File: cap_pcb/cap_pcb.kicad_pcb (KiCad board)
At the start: 2 copper layers, 43 parts, among them U0 ATtiny85-20PU, U1 PCF8574, U10 HDSP-7803, U11 HDSP-7803, U12 PCF8574, U2 HDSP-7803, U3 PCF8574, U4 HDSP-7803, U5 PCF8574, U6 HDSP-7803, U7 PCF8574, U8 HDSP-7803, U9 PCF8574

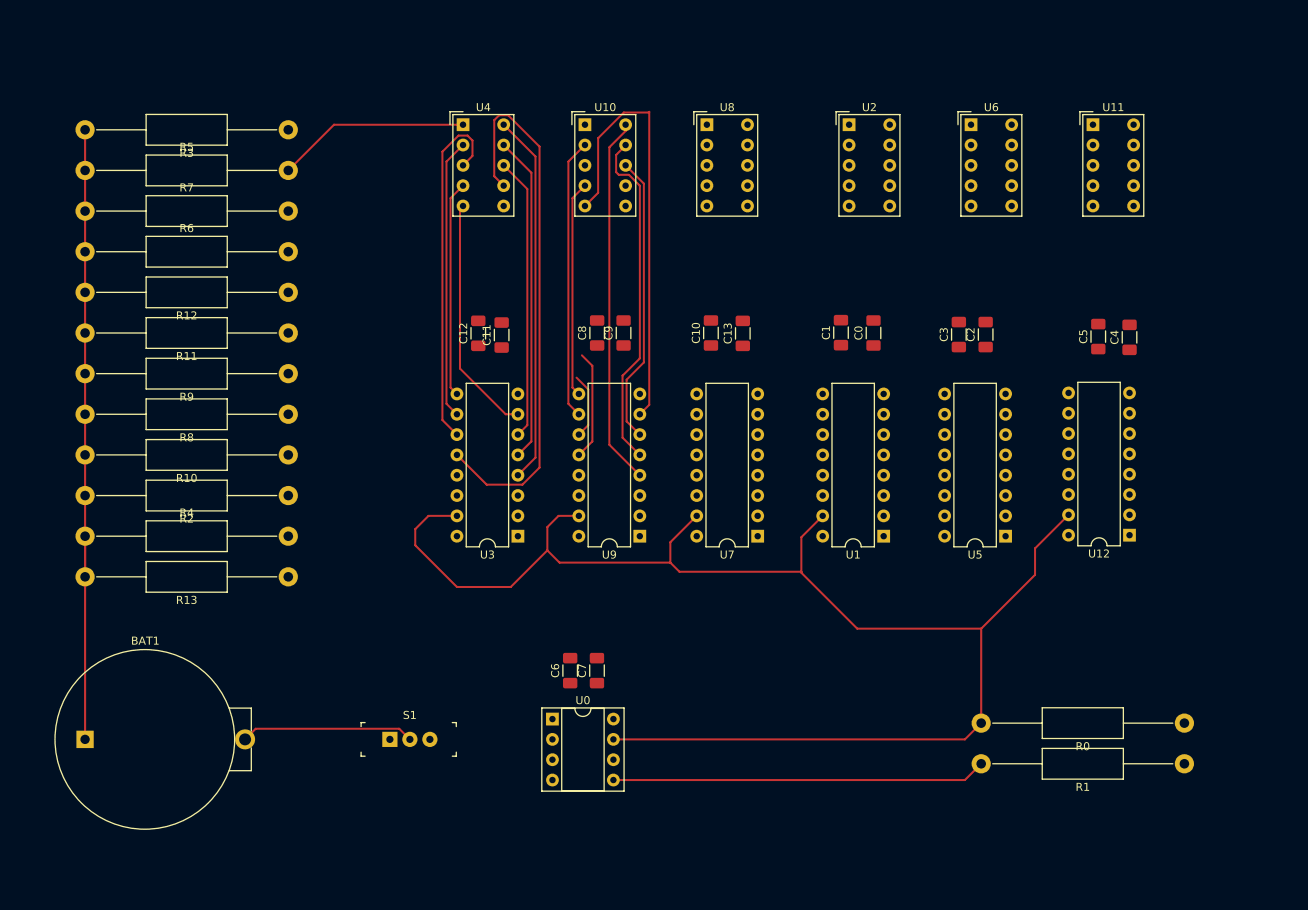
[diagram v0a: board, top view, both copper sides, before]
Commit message: mostly finished pcb
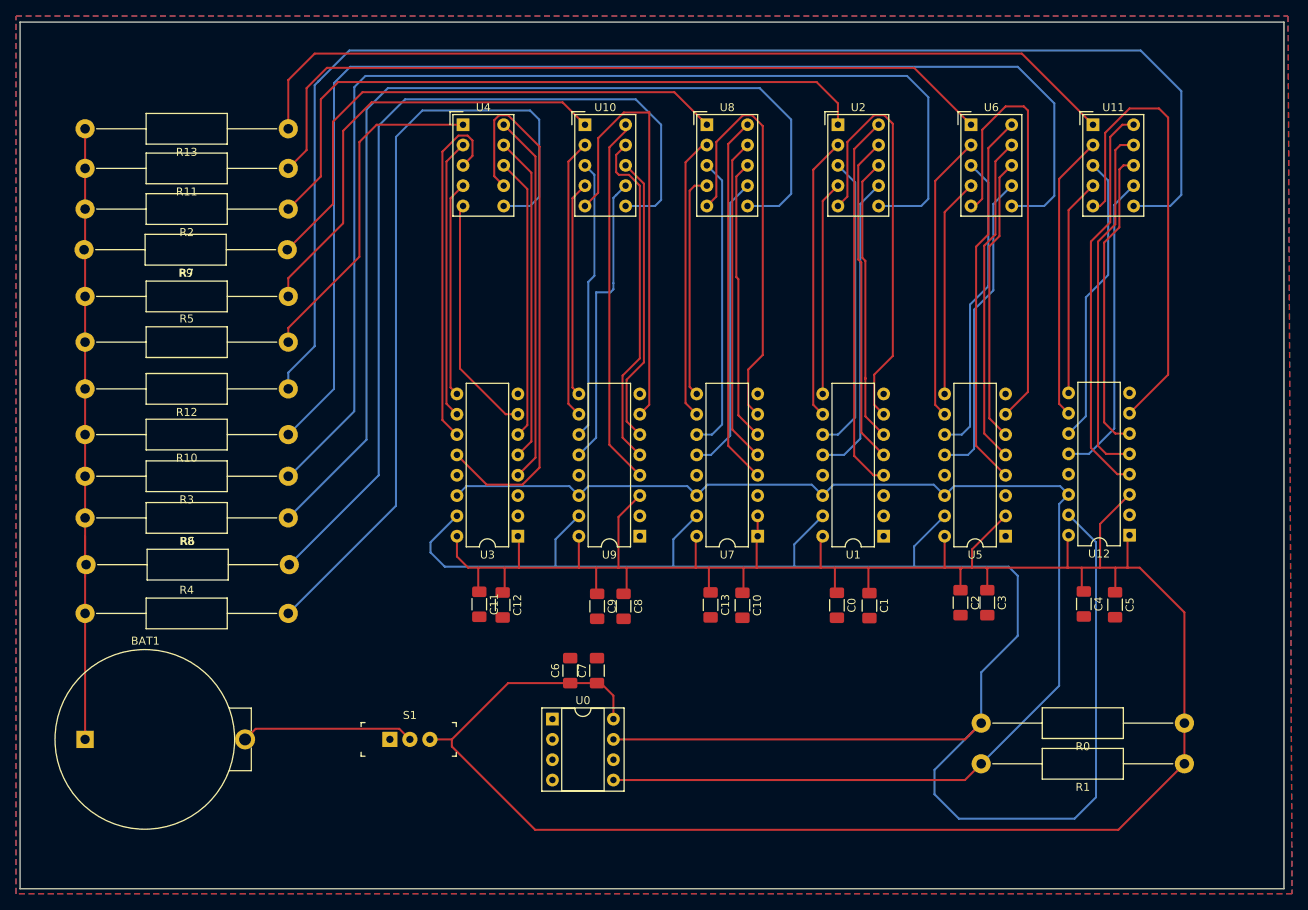
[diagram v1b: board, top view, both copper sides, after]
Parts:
- moved R13 56.0 mm to (106.7, 32.9)
- moved R3 43.3 mm to (106.7, 76.3)
- moved R6 39.1 mm to (81.4, 87.4)
- moved R2 35.8 mm to (106.7, 42.9)
- moved C0 34.3 mm to (175.3, 92.5), turned to 270 degrees
- moved C8 34.3 mm to (148.6, 92.6), turned to 270 degrees
- moved C9 34.3 mm to (145.3, 92.6), turned to 270 degrees
- moved C1 34.3 mm to (179.3, 92.5), turned to 270 degrees
- moved C10 34.3 mm to (163.4, 92.5), turned to 270 degrees
- moved C13 34.2 mm to (159.5, 92.4), turned to 270 degrees
- moved C12 34.1 mm to (133.5, 92.4), turned to 270 degrees
- moved C4 33.8 mm to (206.1, 92.3), turned to 270 degrees
- moved C11 33.8 mm to (130.6, 92.3), turned to 270 degrees
- moved C3 33.7 mm to (194.1, 92.1), turned to 270 degrees
- moved C2 33.7 mm to (190.7, 92.1), turned to 270 degrees
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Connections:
- U5 pad 15: Net-(R1-Pad2) -> Net-(R0-Pad2)
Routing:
- net VCC: track 0.08 -> 346.8 mm
- net Net-(R12-Pad1): track 0.00 -> 171.3 mm
- net Net-(R10-Pad1): track 0.00 -> 156.5 mm
- net Net-(R3-Pad1): track 0.00 -> 144.7 mm
- net Net-(R8-Pad1): track 0.00 -> 126.3 mm
- net Net-(R1-Pad2): track 47.3 -> 167.1 mm
- net Net-(R13-Pad1): track 0.00 -> 111.7 mm
- net Net-(R6-Pad2): track 0.00 -> 111.6 mm
- net Net-(R4-Pad2): track 0.00 -> 99.5 mm
- net Net-(R11-Pad1): track 0.00 -> 98.0 mm
- net Net-(R2-Pad1): track 0.00 -> 84.7 mm
- net Net-(R9-Pad1): track 0.00 -> 68.3 mm
- net Net-(R0-Pad2): track 186.9 -> 249.1 mm
- net Net-(U11-Pad5): track 0.00 -> 58.9 mm
- net Net-(U5-Pad7): track 0.00 -> 56.7 mm
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- added copper zone on B.Cu, net GND
- added copper zone on F.Cu, net GND
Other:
- board outline added: 158 x 108.3 mm
